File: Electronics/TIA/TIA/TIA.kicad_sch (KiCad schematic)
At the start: 3 parts

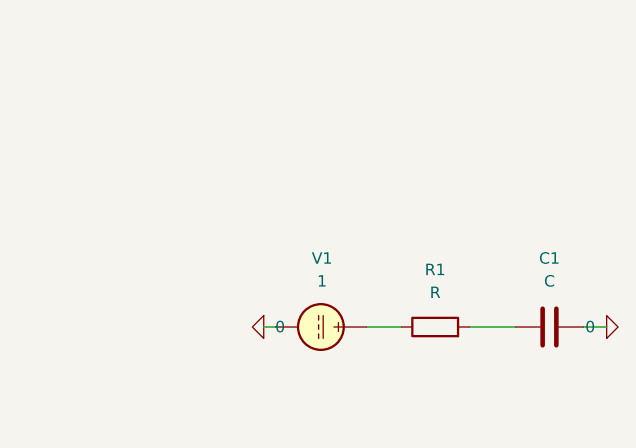
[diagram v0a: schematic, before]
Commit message: Break the simulation somehow
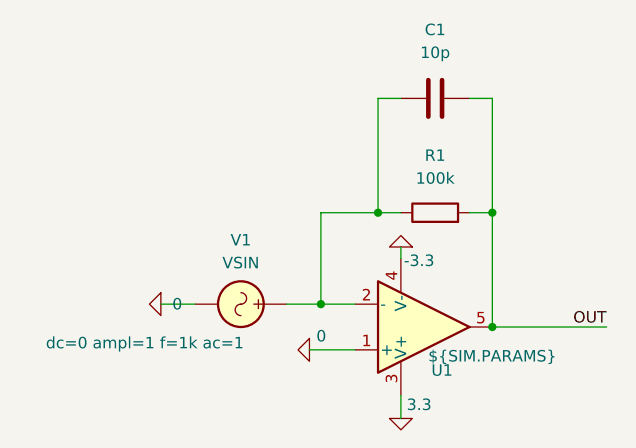
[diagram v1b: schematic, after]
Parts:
- removed V1: 1, symbol Simulation_SPICE:VDC
- added U1: ${SIM.PARAMS}, symbol Simulation_SPICE:OPAMP
- added V1: VSIN, symbol Simulation_SPICE:VSIN
- C1: value C -> 10p
- R1: value R -> 100k
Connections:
- net 0: now also U1.1 (+), V1.2; no longer C1.2
- net at R1.1: now also C1.1, U1.2 (-), V1.1
- net OUT: now reaches R1.2
- net OUT: now also C1.2, U1.5; no longer C1.1
- new net -3.3: U1.4 (V-)
- new net 3.3: U1.3 (V+)
